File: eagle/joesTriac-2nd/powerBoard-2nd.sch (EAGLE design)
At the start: 31 parts, among them IC1 7809, IC2 7805, IC3 7909, IC5 7809, J1 XF2E-0815-1, J2 XF2E-0815-1

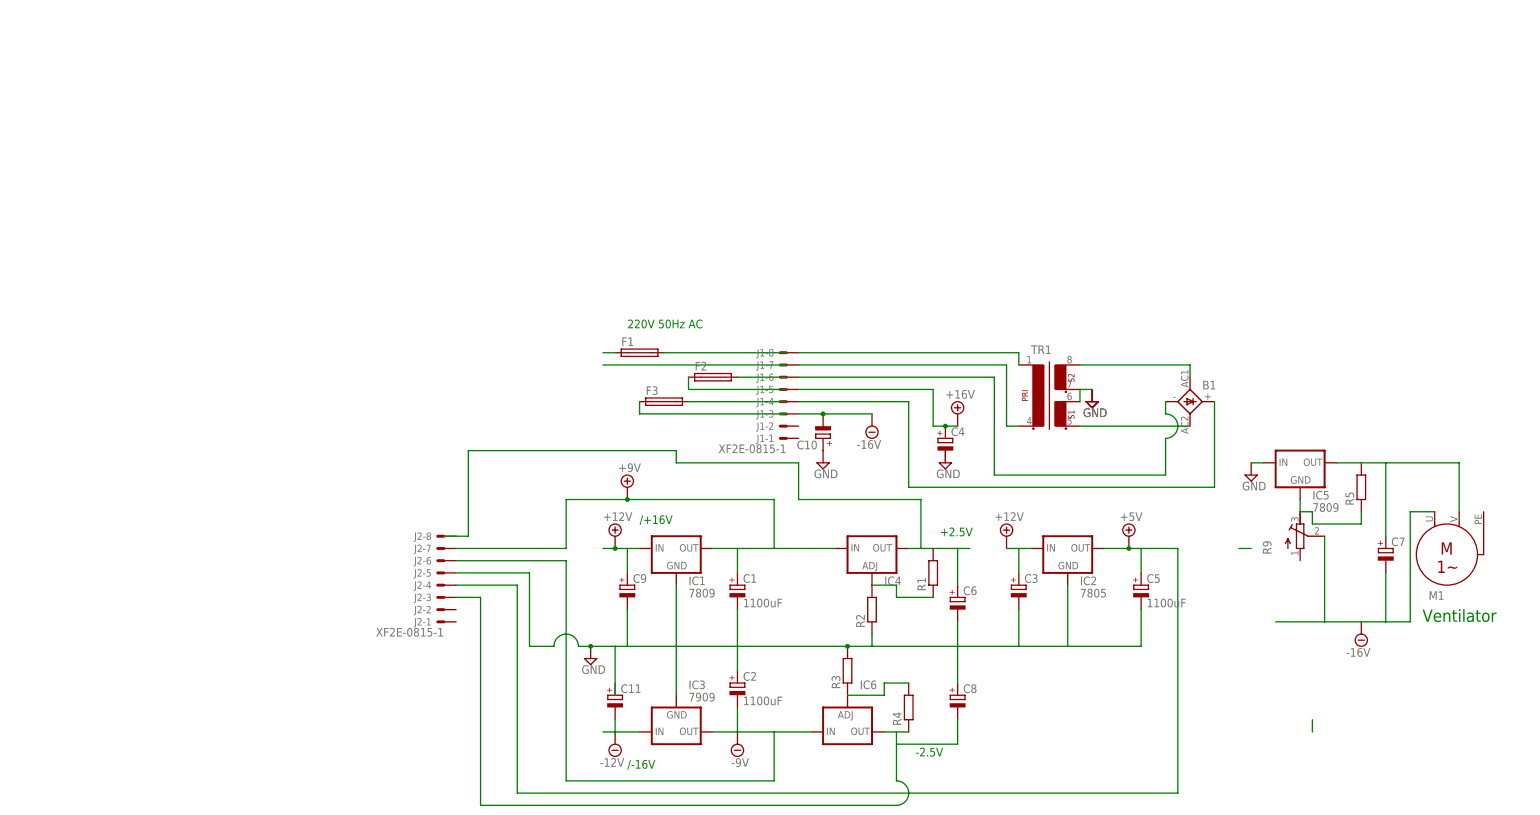
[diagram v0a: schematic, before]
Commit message: reg save
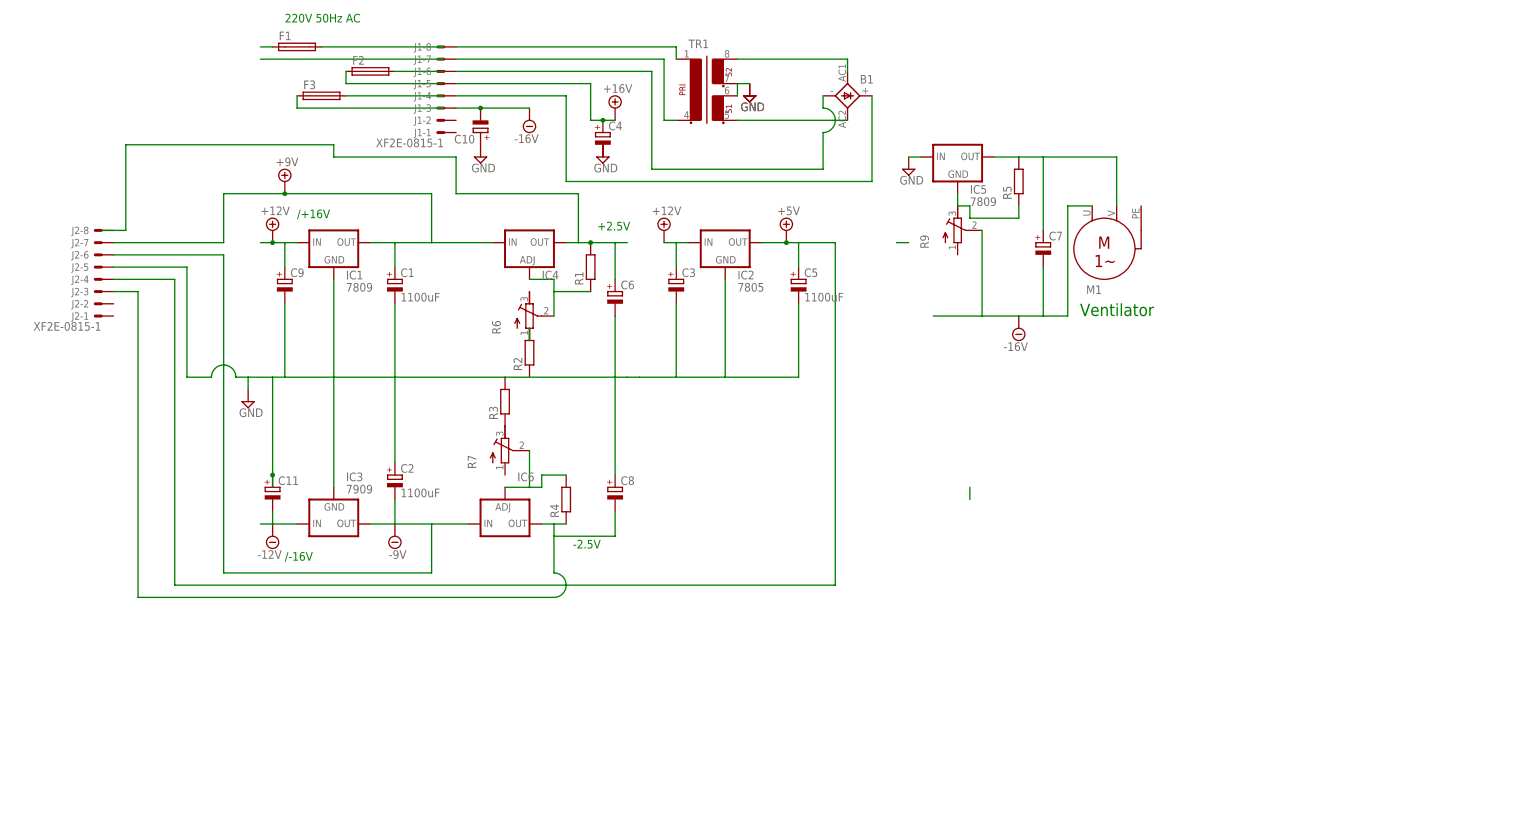
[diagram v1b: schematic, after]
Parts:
- added R6, R7: (no value), resistor:R-TRIMM4G/J
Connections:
- new net N$10: R3.1, R7.E
- new net N$20: IC6.ADJ, R4.2, R7.S
- net GND: now also C11.+; no longer R2.1
- net N$18: now also R6.S; no longer R2.2
- net N$19: now also R2.2, R6.A; no longer IC6.ADJ, R3.1, R4.2
- net N$23: now also R1.2
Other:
- moved on the sheet: B1, C1, C10, C11, C2, C3, C4, C5, C6, C7, C8, C9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
